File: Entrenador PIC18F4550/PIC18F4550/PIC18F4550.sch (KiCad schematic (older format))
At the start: 31 parts, among them J1 Barrel_Jack_Switch, J10 PORTA, J11 PORTC, J12 UART_TTL, J2 Alimenatciones, J3 PICKIT, J5 Conn_01x03_Male, J6 USB_B, J7 PORTE, J8 PORTB, J9 PORTD, SW1 RESET, U1 KA378R33, U2 L7805, U3 PIC18F4550-IP, Y1 Crystal

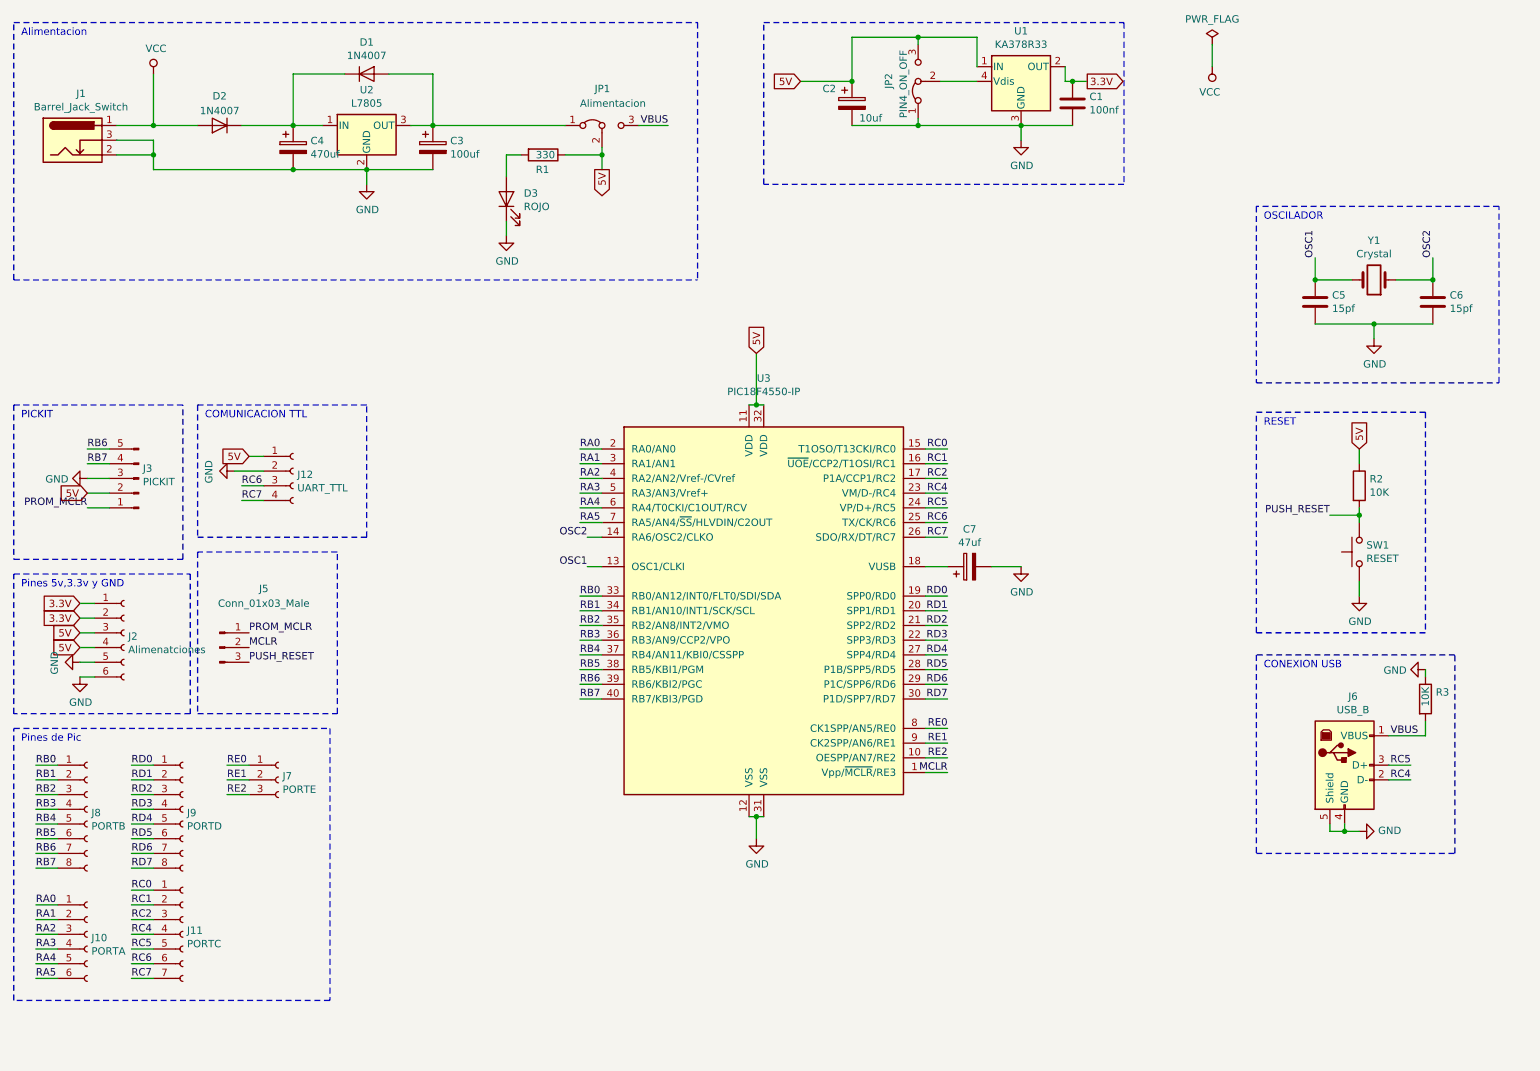
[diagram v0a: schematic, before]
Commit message: Pcbs
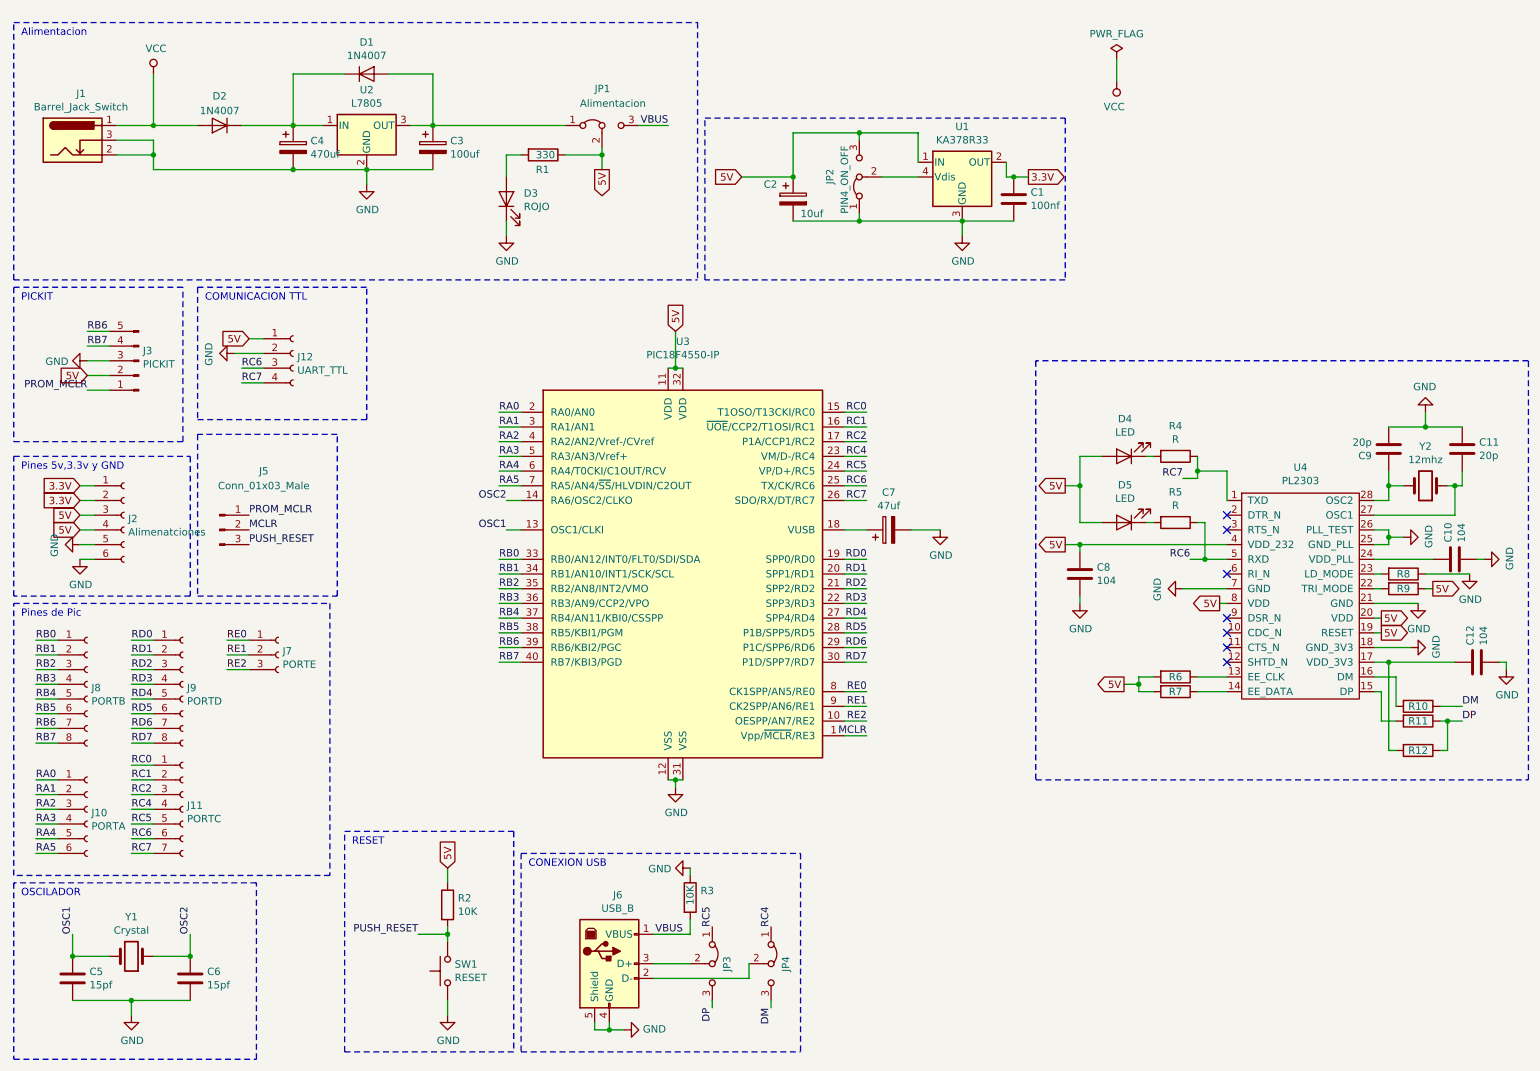
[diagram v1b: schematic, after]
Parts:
- added C10, C12, C8: 104, symbol Device:C
- added C11, C9: 20p, symbol Device:C
- added D4, D5: LED, symbol Device:LED
- added JP3, JP4: Alimentacion, Connector_PinHeader_2.54mm:PinHeader_1x03_P2.54mm_Vertical, symbol Jumper:Jumper_3_Bridged12
- added R10, R11, R4, R5, R6: R, symbol Device:R
- added R12: 1.5k, symbol Device:R
- added R7, R8, R9: 10k, symbol Device:R
- added U4: PL2303, symbol pico_rp2040:PL2303
- added Y2: 12mhz, Crystal:Crystal_HC49-4H_Vertical, symbol Device:Crystal
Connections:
- net 5V: now also C8.2, D4.2 (A), D5.2 (A), R6.2, R7.2, R9.1, U4.19 (RESET), U4.20 (VDD), U4.4 (VDD_232), U4.8 (VDD)
- net GND: now also C10.2, C11.2, C12.2, C8.1, C9.1, R8.1, U4.18 (GND_3V3), U4.21 (GND), U4.25 (GND_PLL), U4.26 (PLL_TEST), U4.7 (GND)
- net RC4: now also JP4.1 (A); no longer J6.2 (D-)
- net RC5: now also JP3.1 (A); no longer J6.3 (D+)
- net RC6: now also R5.1, U4.5 (RXD)
- net RC7: now also R4.1, U4.1 (TXD)
- new net: J6.2 (D-), JP4.2 (C)
- new net: J6.3 (D+), JP3.2 (C)
- new net: R6.1, U4.13 (EE_CLK)
- new net: R7.1, U4.14 (EE_DATA)
- new net: R11.2, U4.15 (DP)
- new net: R10.2, U4.16 (DM)
- new net: C12.1, R12.2, U4.17 (VDD_3V3)
- new net: R9.2, U4.22 (TRI_MODE)
- new net: R8.2, U4.23 (LD_MODE)
- new net: C10.1, U4.24 (VDD_PLL)
- new net: C11.1, U4.27 (OSC1), Y2.1
- new net: C9.2, U4.28 (OSC2), Y2.2
- new net: D4.1 (K), R4.2
- new net: D5.1 (K), R5.2
- new net DM: JP4.3 (B), R10.1
- new net DP: JP3.3 (B), R11.1, R12.1
- no-connect marks 0 -> 7
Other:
- moved on the sheet: C1, C2, C5, C6, C7, J10, J11, J12, J2, J3, J5, J6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
